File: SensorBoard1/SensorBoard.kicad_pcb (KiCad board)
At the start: 2 copper layers, 34.4 x 31.6 mm, 29 parts, among them U1 CE_HEADER, U2 DS7505, U3 74HC595-PWR

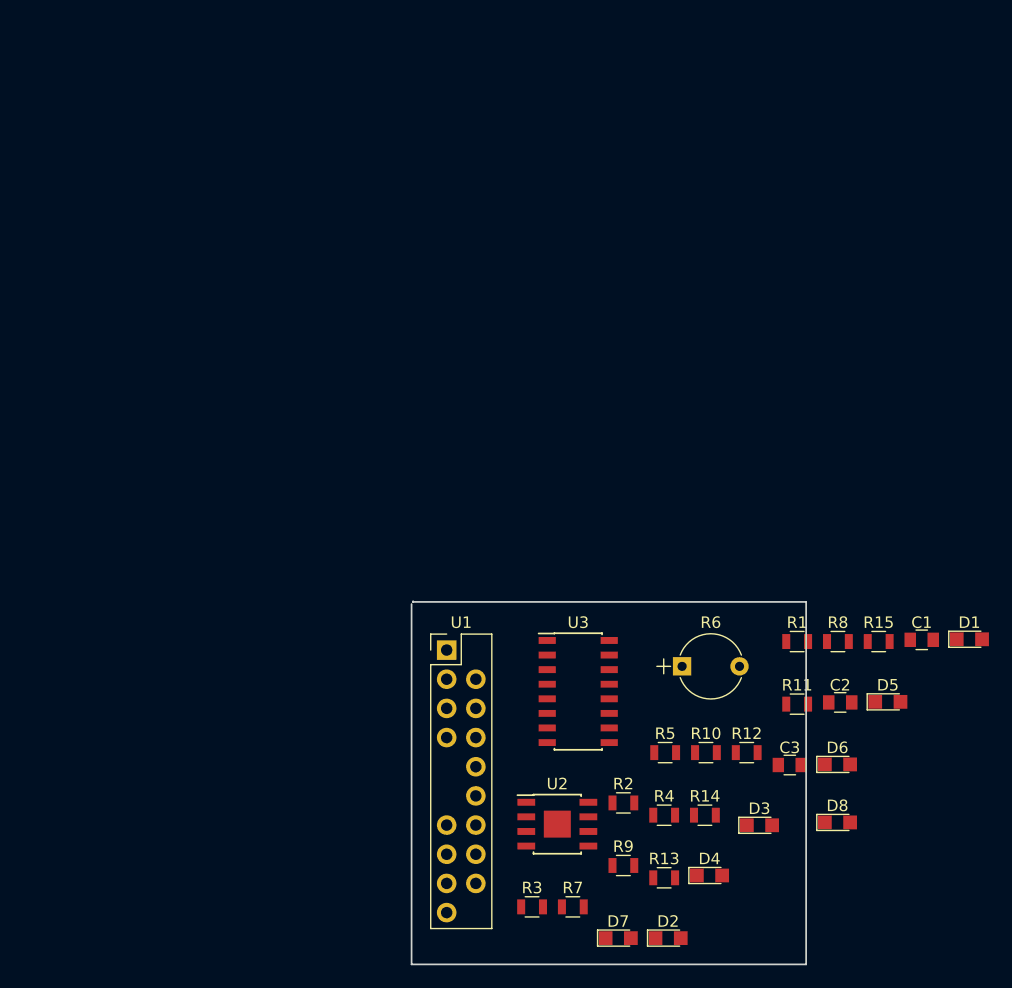
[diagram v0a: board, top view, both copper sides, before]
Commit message: Finished 1.0 Layout
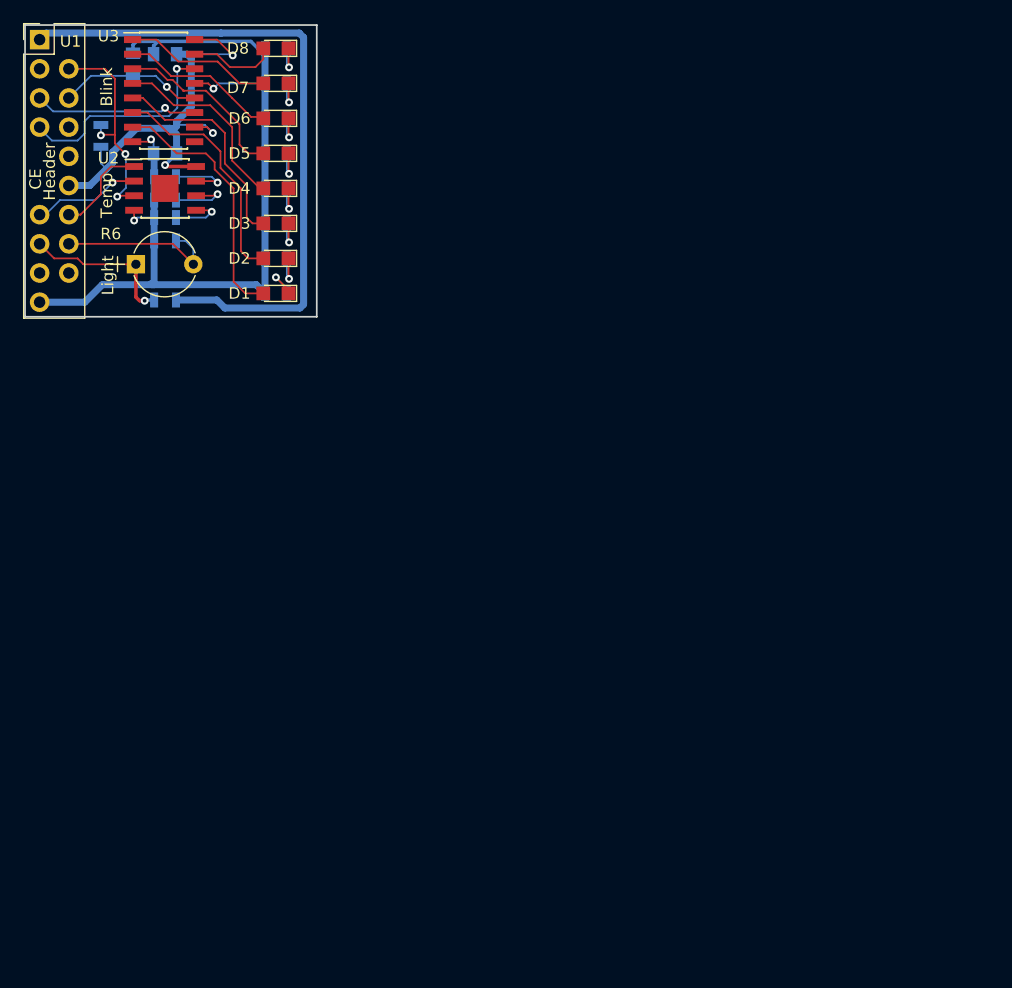
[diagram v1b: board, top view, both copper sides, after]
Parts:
- C1, C2, C3, R1, R10, R11, R12, R13, R14, R15, R2, R3, R4, R5, R7, R8, R9: moved to B.Cu
- moved C1 85.0 mm to (133.9, 56.8), turned to 90 degrees
- moved D8 83.3 mm to (146.3, 55.4), turned to 180 degrees
- moved C3 82.4 mm to (136.7, 55.9)
- moved D7 80.2 mm to (146.3, 58.4), turned to 180 degrees
- moved C2 75.8 mm to (136.7, 64.5)
- moved R1 74.9 mm to (131.1, 63.0), turned to 90 degrees
- moved D6 74.5 mm to (146.3, 61.5), turned to 180 degrees
- moved R13 74.3 mm to (146.3, 61.5), turned to 180 degrees
- moved R14 73.9 mm to (146.3, 58.4), turned to 180 degrees
- moved R15 73.6 mm to (146.3, 55.4), turned to 180 degrees
- moved D5 71.5 mm to (146.3, 64.5), turned to 180 degrees
- moved D4 70.7 mm to (146.3, 67.6), turned to 180 degrees
- moved R4 70.6 mm to (136.7, 66.5), turned to 180 degrees
- moved R3 69.3 mm to (136.7, 68.6), turned to 180 degrees
- moved D2 68.3 mm to (146.3, 73.7), turned to 180 degrees
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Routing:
- net GND: track 0.00 -> 80.1 mm, vias 0 -> 3
- net /5V: track 0.00 -> 58.2 mm
- net /3.3V: track 0.00 -> 42.6 mm, vias 0 -> 3
- net Net-(D1-Pad2): track 0.00 -> 22.5 mm
- net Net-(D2-Pad2): track 0.00 -> 20.7 mm
- net /dataPin: track 0.00 -> 19.3 mm, vias 0 -> 1
- net Net-(D3-Pad2): track 0.00 -> 19.1 mm
- net /O.S.: track 0.00 -> 19.0 mm, vias 0 -> 3
- net Net-(D4-Pad2): track 0.00 -> 16.9 mm
- net Net-(D5-Pad2): track 0.00 -> 15.5 mm
- net /PR_BOT: track 0.00 -> 14.7 mm
- net /clockPin: track 0.00 -> 14.3 mm, vias 0 -> 1
- net /PR_TOP: track 0.00 -> 13.7 mm, vias 0 -> 1
- net Net-(D6-Pad2): track 0.00 -> 13.7 mm
- net Net-(D7-Pad2): track 0.00 -> 13.0 mm
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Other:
- board size 34.4 x 31.6 mm -> 25.4 x 25.4 mm
- net class Default: clearance 0.2 -> 0.1524; trace_width 0.25 -> 0.1524; via_dia 0.6 -> 0.6858; via_drill 0.4 -> 0.3302
- rule trace_clearance: 0.2 -> 0.1524
- rule trace_min: 0.2 -> 0.1524
- rule via_min_drill: 0.3 -> 0.3302
- rule via_min_size: 0.4 -> 0.6858
- board text added: "Blink"
- board text added: "CE"
- board text added: "Header"
- board text added: "Light"
- board text added: "Temp"
